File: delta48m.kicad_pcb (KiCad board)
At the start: 2 copper layers, 287 x 150 mm, 198 parts, among them J1 SNP, J2 DIN-7 Video, J3 DIN-5 Audio, J4 DIN-5 Power, J5 Keyboard Connector, J6 Joystick 1, J7 Joystick 2, J8 RGB/Composite, Q1 BC547B, Q3 BC547B, Q4 BC547B, Q5 BC547B, Q6 BC547B, Q7 BC547B, Q8 BC547B, SW1 Reset button, U1 SN74ALS08 (КР1533ЛИ1), U10 SN74ALS08 (КР1533ЛИ1), U11 IN74ALS00N (КР1533ЛА3), U12 IN74ALS02N (КР1533ЛЕ1), U13 SN74ALS10 (КР1533ЛА4), U14 SN74ALS86N (КР1533ЛП5), U15 CD4520АN_(К561ИЕ10), U16 SN74ALS257N_(КР1533КП11А), U17 CD4520АN_(К561ИЕ10), U18 CD4011 (К561ЛА7), U19 SN74ALS04 (КР1533ЛН1), U2 SN74ALS04 (КР1533ЛН1), U20 SN74ALS74AN (КР1533ТМ2), U21 SN74ALS14 (КР1533ТЛ2), U22 74LS257 (КР1533КП11А), U23 SN74ALS253N (КР1533КП12), U24 SN74ALS253N (КР1533КП12), U25 74LS257 (КР1533КП11А), U26 SN74ALS253N (КР1533КП12), U27 SN74ALS253N (КР1533КП12), U28 IN74ALS32N (КР1533ЛЛ1), U29 IN74ALS32N (КР1533ЛЛ1), U3 SN74ALS74AN (КР1533ТМ2), U30 IN74ALS02N (КР1533ЛЕ1), U31 RU5D1, U32 RU5D1, U33 RU5D1, U34 RU5D1, U35 RU5D1, U36 RU5D1, U37 RU5D1, U38 RU5D1, U39 IN74ALS32N (КР1533ЛЛ1), U4 SN74ALS193N_(КР1533ИЕ7), U40 IN74ALS00N (КР1533ЛА3), U41 2118 (КР565РУ6), U42 2118 (КР565РУ6), U43 2118 (КР565РУ6), U44 2118 (КР565РУ6), U45 2118 (КР565РУ6), U46 2118 (КР565РУ6), U47 2118 (КР565РУ6), U48 2118 (КР565РУ6), U49 SN74ALS04 (КР1533ЛН1), U5 СD4013АN_(К561ТМ2), U50 SN74ALS86N (КР1533ЛП5), U51 SN7486N (К155ЛП5), U52 SN74ALS175N (КР1533ТМ8), U53 SN74ALS153N (КР1533КП2), U54 SN74ALS298N (КР1533КП13), U55 74LS257 (КР1533КП11А), U56 SN74ALS175N_U56, U57 SN74LS295N_(К555ИР16), U58 SN74LS295N_(К555ИР16), U59 SN74ALS175N (КР1533ТМ8), U6 CD4015A (К561ИР2), U60 SN74ALS153N (КР1533КП2), U61 SN74ALS298N (КР1533КП13), U62 74LS257 (КР1533КП11А), U63 SN74ALS175N_U63, U64 SN74LS295N_(К555ИР16), U65 SN74LS295N_(К555ИР16), U66 SN74ALS175N (КР1533ТМ8), U67 8282 (КР580ИР82)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

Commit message: 28th march ver2
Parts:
- added C26: 0.1μF, Capacitor_THT:C_Disc_D7.0mm_W2.5mm_P5.00mm, F.Cu at (335.0, 144.9)
- added C27: 0.1μF, Capacitor_THT:C_Disc_D7.0mm_W2.5mm_P5.00mm, F.Cu at (335.0, 123.0)
- RV42, RV43, RV44: footprint Potentiometer_THT:Potentiometer_Bourns_3296X_Horizontal -> Potentiometer_THT:Potentiometer_Bourns_3299X_Horizontal
- moved C3 40.3 mm to (77.3, 155.5), turned to -90 degrees
- moved Y1 38.5 mm to (76.4, 117.2), turned to 0 degrees
- moved R2 36.5 mm to (73.4, 111.8), turned to 90 degrees
- moved C32 33.2 mm to (87.8, 106.8)
- moved C8 26.8 mm to (113.4, 160.0)
- moved R8 24.3 mm to (110.6, 113.5)
- moved C1 22.8 mm to (78.5, 106.7), turned to 90 degrees
- moved R7 21.9 mm to (98.3, 97.3), turned to 0 degrees
- moved R6 21.0 mm to (81.2, 176.7)
- moved U66 19.4 mm to (280.5, 167.8), turned to 180 degrees
- moved RV42 19.1 mm to (272.2, 79.1)
- moved R9 18.6 mm to (110.9, 133.9)
- moved R4 12.9 mm to (81.3, 152.8)
- moved R5 11.7 mm to (81.2, 149.4)
- moved R1 11.0 mm to (83.6, 101.6), turned to -90 degrees
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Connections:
- U1 pad 12: Net-(R8-Pad1) -> Net-(U13-Pad12)
- U1 pad 13: Net-(U1-Pad13) -> Net-(R8-Pad1)
- U13 pad 12: Net-(U1-Pad13) -> Net-(U13-Pad12)
- U3 pad 12: Net-(U1-Pad13) -> Net-(U13-Pad12)
- U49 pad 1: unconnected-(U49-Pad1) -> Net-(U10-Pad3)
- U49 pad 2: unconnected-(U49-Pad2) -> ТАКТ
- U49 pad 3: Net-(U10-Pad3) -> unconnected-(U49-Pad3)
- U49 pad 4: ТАКТ -> unconnected-(U49-Pad4)
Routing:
- net Contact2: track 238.6 -> 344.1 mm, vias 5 -> 6
- net JOY4: track 306.3 -> 406.5 mm
- net Net-(U10-Pad3): track 203.3 -> 296.0 mm, vias 4 -> 5
- net A14: track 411.2 -> 498.7 mm, vias 4 -> 3
- net A19_SNP: track 0.00 -> 87.4 mm, vias 0 -> 1
- net ZPVDN: track 281.4 -> 363.4 mm, vias 2 -> 4
- net Net-(R10-Pad1): track 98.2 -> 177.7 mm, vias 2 -> 4
- net ADR3: track 215.2 -> 141.8 mm
- net A10: track 348.3 -> 419.0 mm, vias 4 -> 5
- net Net-(U1-Pad13): track 62.3 -> 0.00 mm, vias 1 -> 0
- net Net-(U13-Pad12): track 0.00 -> 56.0 mm
- net ADR7: track 137.5 -> 185.4 mm, vias 2 -> 1
- net D0: track 307.5 -> 353.3 mm, vias 5 -> 4
- net ЧТL: track 285.4 -> 330.8 mm, vias 3 -> 5
- net +5V: track 1519.4 -> 1562.5 mm, vias 1 -> 2
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
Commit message: 29th march 2023 Update 1
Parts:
- moved R45 11.4 mm to (271.3, 128.1), turned to -90 degrees
- moved R46 11.4 mm to (274.6, 128.1), turned to -90 degrees
- moved R51 11.0 mm to (299.7, 165.6), turned to -90 degrees
- moved R35 10.2 mm to (254.6, 113.3), turned to 90 degrees
- moved R50 2.56 mm to (296.2, 165.6)
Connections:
- R55 pad 2: Net-(R55-Pad2) -> Net-(U66-Pad7)
- U16 pad 13: CT9 -> Net-(U16-Pad13)
- U16 pad 2: Net-(U16-Pad2) -> CT9
- U16 pad 5: CT9 -> Net-(U16-Pad13)
- U17 pad 5: CT9 -> Net-(U16-Pad13)
- U17 pad 6: Net-(U16-Pad2) -> CT9
- U18 pad 5: CT9 -> Net-(U16-Pad13)
- U18 pad 6: Net-(U16-Pad2) -> CT9
- U66 pad 14: Net-(R55-Pad2) -> unconnected-(U66-Pad14)
- U66 pad 7: unconnected-(U66-Pad7) -> Net-(U66-Pad7)
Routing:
- net Net-(U66-Pad7): track 0.00 -> 120.1 mm, vias 0 -> 1
- net JOY4: track 406.5 -> 289.8 mm, vias 2 -> 3
- net Net-(R55-Pad2): track 104.5 -> 0.00 mm, vias 4 -> 0
- net ZPVDN: track 363.4 -> 267.4 mm, vias 4 -> 2
- net ПРL: track 421.7 -> 327.6 mm, vias 1 -> 2
- net Contact2: track 344.1 -> 254.5 mm
- net Net-(U10-Pad3): track 296.0 -> 233.3 mm, vias 5 -> 3
- net RASL: track 193.2 -> 134.0 mm, vias 4 -> 2
- net MUX_S: track 173.1 -> 118.5 mm, vias 7 -> 1
- net ADR7: track 185.4 -> 134.8 mm, vias 1 -> 0
- net A14: track 498.7 -> 451.5 mm, vias 3 -> 7
- net Net-(R10-Pad1): track 177.7 -> 130.5 mm, vias 4 -> 6
- net A1: track 332.3 -> 378.0 mm, vias 5 -> 6
- net A13: track 383.3 -> 427.1 mm, vias 4 -> 3
- net ЧТL: track 330.8 -> 291.9 mm, vias 5 -> 3
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
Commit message: March 31st Update
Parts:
- added C13: 0.1μF, Capacitor_THT:C_Disc_D7.0mm_W2.5mm_P5.00mm, F.Cu at (137.8, 194.9)
- added C16: 0.1μF, Capacitor_THT:C_Disc_D7.0mm_W2.5mm_P5.00mm, F.Cu at (191.8, 183.5)
- added C17: 0.1μF, Capacitor_THT:C_Disc_D7.0mm_W2.5mm_P5.00mm, F.Cu at (191.8, 200.7)
- added C18: 0.1μF, Capacitor_THT:C_Disc_D7.0mm_W2.5mm_P5.00mm, F.Cu at (219.8, 146.0)
- added C19: 0.1μF, Capacitor_THT:C_Disc_D7.0mm_W2.5mm_P5.00mm, F.Cu at (219.7, 134.5)
- added C2: 0.1μF, Capacitor_THT:C_Disc_D7.0mm_W2.5mm_P5.00mm, F.Cu at (87.6, 135.6)
- added C20: 0.1μF, Capacitor_THT:C_Disc_D7.0mm_W2.5mm_P5.00mm, F.Cu at (217.7, 194.9)
- added C23: 0.1μF, Capacitor_THT:C_Disc_D7.0mm_W2.5mm_P5.00mm, F.Cu at (271.3, 146.0)
- added C24: 0.1μF, Capacitor_THT:C_Disc_D7.0mm_W2.5mm_P5.00mm, F.Cu at (267.8, 194.9)
- added C29: 0.1μF, Capacitor_THT:C_Disc_D7.0mm_W2.5mm_P5.00mm, F.Cu at (332.6, 193.1)
- added C30: 0.1μF, Capacitor_THT:C_Disc_D7.0mm_W2.5mm_P5.00mm, F.Cu at (354.5, 198.1)
- added C31: 0.1μF, Capacitor_THT:C_Disc_D7.0mm_W2.5mm_P5.00mm, F.Cu at (167.5, 193.4)
- added C9: 0.1μF, Capacitor_THT:C_Disc_D7.0mm_W2.5mm_P5.00mm, F.Cu at (112.1, 194.9)
- moved J7 31.8 mm to (150.1, 84.2)
- moved U70 20.3 mm to (330.0, 119.5)
- moved U71 20.3 mm to (330.0, 139.8)
- moved RV44 18.9 mm to (307.3, 79.0)
- moved J2 11.6 mm to (233.4, 84.2)
- moved J4 11.4 mm to (212.6, 84.2)
- moved JP3 11.4 mm to (163.7, 197.6)
- moved J3 11.2 mm to (191.8, 84.2)
- moved R57 11.1 mm to (347.3, 214.2), turned to 180 degrees
- moved R16 10.6 mm to (153.7, 202.7)
- moved RV43 10.4 mm to (290.8, 79.0)
- moved J6 10.4 mm to (170.9, 84.2)
- moved C25 10.4 mm to (290.4, 139.1), turned to 180 degrees
- moved D22 10.2 mm to (299.6, 182.6), turned to -90 degrees
- moved D23 10.2 mm to (302.1, 182.6), turned to -90 degrees
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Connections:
- U56 pad 10: Net-(U54-Pad1) -> Net-(U54-Pad5)
- U56 pad 15: Net-(U54-Pad5) -> Net-(U54-Pad1)
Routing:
- net JOY3: track 288.0 -> 399.0 mm, vias 4 -> 0
- net JOY5: track 286.5 -> 387.0 mm
- net JOY4: track 289.8 -> 383.5 mm, vias 3 -> 0
- net 7MHZ: track 322.4 -> 409.7 mm, vias 5 -> 1
- net ПРL: track 327.6 -> 410.5 mm, vias 2 -> 1
- net A14: track 451.5 -> 381.2 mm
- net Net-(U10-Pad3): track 233.3 -> 299.2 mm, vias 3 -> 2
- net A11: track 441.4 -> 377.1 mm, vias 5 -> 6
- net Net-(U10-Pad13): track 168.7 -> 104.5 mm, vias 1 -> 3
- net Net-(U39-Pad1): track 32.2 -> 86.7 mm, vias 0 -> 1
- net GND: track 1791.3 -> 1845.4 mm
- net ZPRGBD: track 264.9 -> 309.7 mm, vias 3 -> 2
- net A10: track 390.2 -> 346.6 mm, vias 4 -> 3
- net Net-(U19-Pad2): track 220.8 -> 263.3 mm, vias 4 -> 2
- net D2: track 263.1 -> 305.3 mm, vias 3 -> 4
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
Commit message: Version 0.1 (March 31st)
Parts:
- J5: footprint Connector_IDC:IDC-Header_2x12_P2.54mm_Vertical -> delta:Keyboard_connector
- RV42, RV43, RV44: footprint Potentiometer_THT:Potentiometer_Bourns_3299X_Horizontal -> delta:Potentiometer_3299X
- U56: value SN74ALS175N_U56 -> SN74ALS175N (КР1533ТМ8)
- U63: value SN74ALS175N_U63 -> SN74ALS175N (КР1533ТМ8)
- moved R8 0.13 mm to (110.7, 113.5)
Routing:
- net Contact2: track 293.1 -> 302.7 mm
- net GND: track 1845.4 -> 1847.3 mm
- net Down1: track 43.1 -> 43.6 mm
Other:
- board text added: "1"
- board text added: "10K"
- board text added: "2"
- board text added: "2118 (КР565РУ6)"
- board text added: "27C64 (К573РФ4)"
- board text added: "3"
- board text added: "4"
- board text added: "5"
- board text added: "6"
- board text added: "7"
- board text added: "74LS257 (КР1533КП11А)"
- board text added: "8282 (КР580ИР82)"
- board text added: "Blue (Синий)"
- board text added: "CD4011 (К561ЛА7)"
- board text added: "CD4015A (К561ИР2)"
- board text added: "CD4520АN (К561ИЕ10)"
- board text added: "For b/w composite on Video line short 1-2, 3-4, 5-6"
- board text added: "Green (Зеленый)"
- board text added: "IN74ALS00N (КР1533ЛА3)"
- board text added: "IN74ALS02N (КР1533ЛЕ1)"
- board text added: "IN74ALS32N (КР1533ЛЛ1)"
- board text added: "Red (Красный)"
- board text added: "SN7486N (К155ЛП5)"
- board text added: "SN74ALS04 (КР1533ЛН1)"
- board text added: "SN74ALS08 (КР1533ЛИ1)"
- board text added: "SN74ALS10 (КР1533ЛА4)"
- board text added: "SN74ALS14 (КР1533ТЛ2)"
- board text added: "SN74ALS153N (КР1533КП2)"
- board text added: "SN74ALS175N (КР1533ТМ8)"
- board text added: "SN74ALS193N (КР1533ИЕ7)"
- board text added: "SN74ALS253N (КР1533КП12)"
- board text added: "SN74ALS257N (КР1533КП11А)"
- board text added: "SN74ALS298N (КР1533КП13)"
- board text added: "SN74ALS74AN (КР1533ТМ2)"
- board text added: "SN74ALS86N (КР1533ЛП5)"
- board text added: "SN74LS295N (К555ИР16)"
- board text added: "Short 1-2 for 2x 27C64 Short 2-3 for 1x 27C128"
- board text added: "Z80 CPU"
- board text added: "КР556РТ2"
- board text added: "КР565РУ5Д1"
- board text added: "Маркировка диодов выполнена под 1N4148 У КД522Б обозначение катода обратное!"
- board text added: "СD4001АN (К561ЛЕ5)"
- board text added: "СD4013АN (К561ТМ2)"

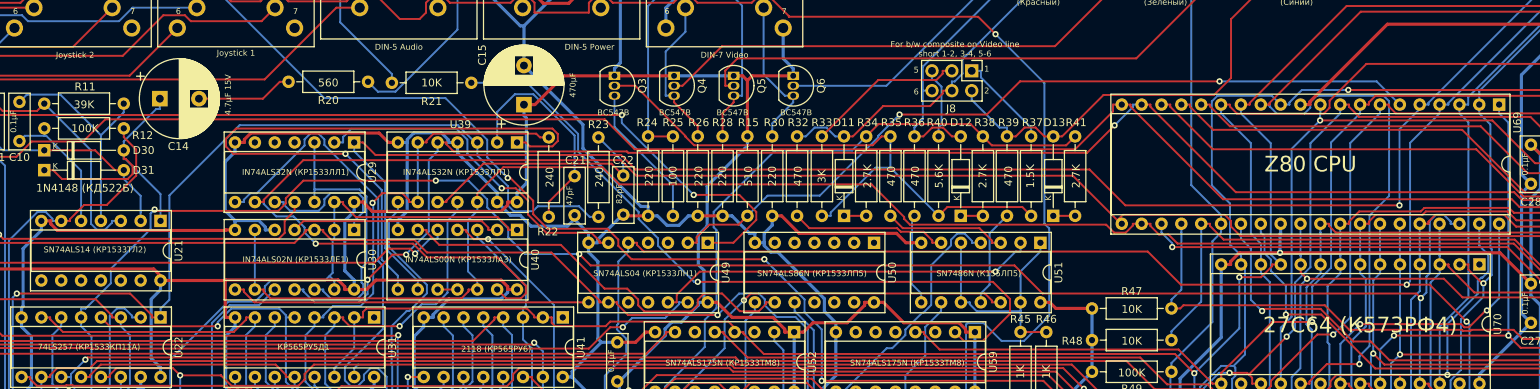
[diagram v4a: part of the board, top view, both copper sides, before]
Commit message: Update delta48m.kicad_pcb
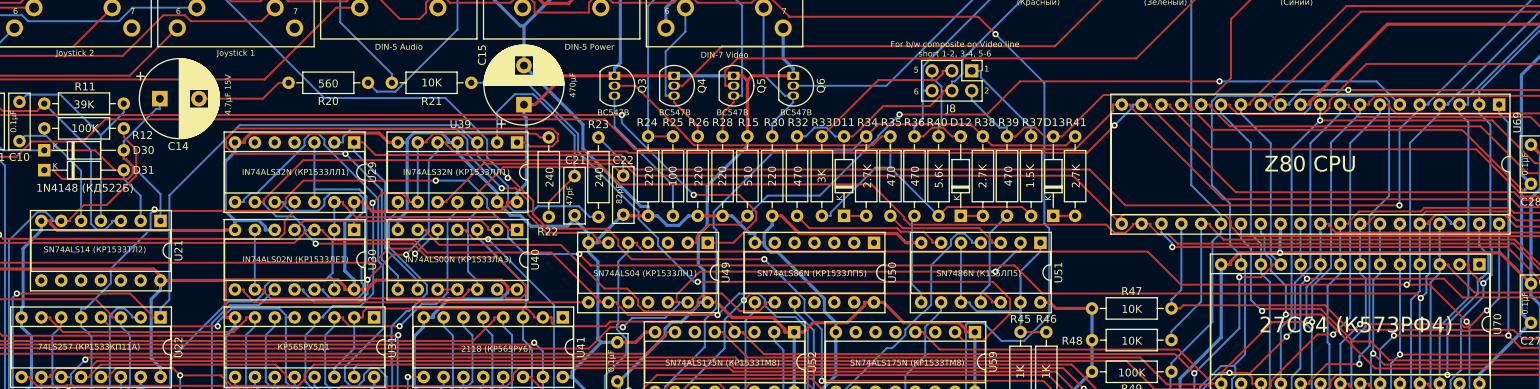
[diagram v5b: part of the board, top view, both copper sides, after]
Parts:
- moved R20 0.13 mm to (187.8, 96.3)
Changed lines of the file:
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@@
   )
   (footprint "Resistor_THT:R_Axial_DIN0207_L6.3mm_D2.5mm_P10.16mm_Horizontal" (layer "F.Cu")
-    (at 187.833 96.139 180)
+    (at 187.833 96.266 180)
     (descr "Resistor, Axial_DIN0207 series, Axial, Horizontal, pin pitch=10.16mm, 0.25W = 1/4W, length*diameter=6.3*2.5mm^2, http://cdn-reichelt.de/documents/datenblatt/B400/1_4W%23YAG.pdf")
     (tags "Resistor Axial_DIN0207 series Axial Horizontal pin pitch 10.16mm 0.25W = 1/4W length 6.3mm diameter 2.5mm")
@@
       (effects (font (size 1 1) (thickness 0.15)))
     )
-    (fp_text value "Joystick 2" (at 0.254 8.549) (layer "F.SilkS")
+    (fp_text value "Joystick 2" (at 0.254 8.295) (layer "F.SilkS")
       (effects (font (size 0.75 0.75) (thickness 0.15)))
     )
@@
     (effects (font (size 0.75 0.75) (thickness 0.15)))
   )
-  (gr_text "27C64 (К573РФ4)" (at 314.706 127.254) (layer "F.SilkS")
+  (gr_text "27C64 (К573РФ4)" (at 314.198 127.254) (layer "F.SilkS")
     (effects (font (size 2 2) (thickness 0.3)))
   )
@@
   (segment (start 160.7448 99.6231) (end 156.591 103.7769) (width 0.25) (layer "B.Cu") (net 14))
   (segment (start 161.295 113.929) (end 161.295 110.498) (width 0.25) (layer "B.Cu") (net 14))
-  (segment (start 166.2083 98.298) (end 174.3889 98.298) (width 0.25) (layer "F.Cu") (net 15))
-  (segment (start 177.673 96.139) (end 176.5479 96.139) (width 0.25) (layer "F.Cu") (net 15))
-  (segment (start 174.3889 98.298) (end 176.5479 96.139) (width 0.25) (layer "F.Cu") (net 15))
+  (segment (start 174.3889 98.298) (end 166.2083 98.298) (width 0.25) (layer "F.Cu") (net 15))
+  (segment (start 176.4209 96.266) (end 174.3889 98.298) (width 0.25) (layer "F.Cu") (net 15))
+  (segment (start 177.673 96.266) (end 176.4209 96.266) (width 0.25) (layer "F.Cu") (net 15))
   (segment (start 160.4237 120.0776) (end 161.8951 121.549) (width 0.4) (layer "F.Cu") (net 16))
   (segment (start 234.3937 126.2696) (end 232.4671 124.343) (width 0.4) (layer "F.Cu") (net 16))
@@
   (segment (start 348.782 111.534) (end 346.282 111.534) (width 0.25) (layer "F.Cu") (net 76))
   (segment (start 335.7776 110.3052) (end 338.5421 110.3052) (width 0.25) (layer "F.Cu") (net 76))
-  (segment (start 187.833 96.139) (end 189.0958 97.4018) (width 0.25) (layer "B.Cu") (net 77))
-  (segment (start 189.0958 97.4018) (end 191.3397 97.4018) (width 0.25) (layer "B.Cu") (net 77))
-  (segment (start 191.3397 97.4018) (end 199.27 89.4715) (width 0.25) (layer "B.Cu") (net 77))
   (segment (start 199.27 89.4715) (end 199.27 84.161) (width 0.25) (layer "B.Cu") (net 77))
+  (segment (start 188.9688 97.4018) (end 191.3397 97.4018) (width 0.25) (layer "B.Cu") (net 77))
+  (segment (start 187.833 96.266) (end 188.9688 97.4018) (width 0.25) (layer "B.Cu") (net 77))
+  (segment (start 191.3397 97.4018) (end 199.27 89.4715) (width 0.25) (layer "B.Cu") (net 77))
   (segment (start 109.9916 95.8347) (end 174.6119 95.8347) (width 0.25) (layer "F.Cu") (net 78))
   (segment (start 99.0871 96.1528) (end 99.0871 96.52) (width 0.25) (layer "F.Cu") (net 78))
